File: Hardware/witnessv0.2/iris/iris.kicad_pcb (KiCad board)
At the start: 4 copper layers, 20 x 40 mm, 96 parts, among them J1 Conn_01x02, J2 Conn_01x02, J3 USB_B_Micro, J4 Conn_01x02, J5 Conn_01x04, J6 Conn_01x04, J7 Conn_01x04, J8 Conn_01x04, Q1 SQA403EJ, Q11 AO3400A, Q12 SQA403EJ, Q2 SQA403EJ, Q3 SQA403EJ, Q4 AO3400A, Q5 AO3400A, Q6 SQA403EJ, U1 PAC1934x-xJQ, U2 ME6118A33PG, U3 LTV-817S, U4 MCP23008-xML, U5 TCAN1044A-Q1, U6 TPS63070, U7 ESP32-C3FH4, U9 USBLC6-2SC6, Y1 F322540MUBCE2O

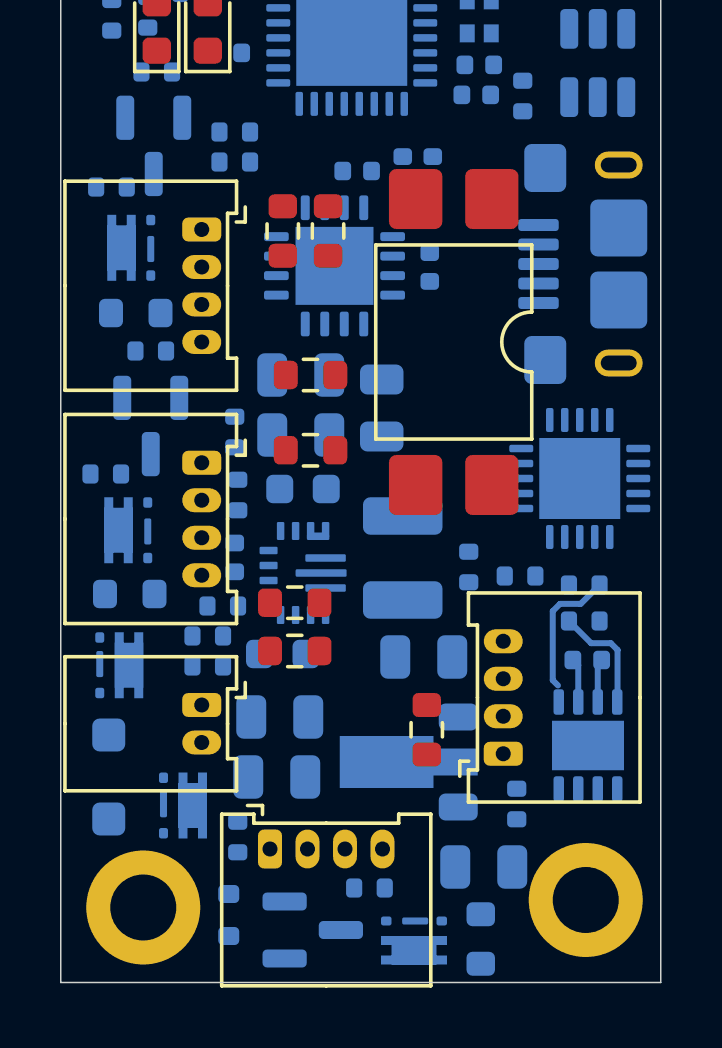
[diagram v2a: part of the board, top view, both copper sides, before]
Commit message: for foo & root
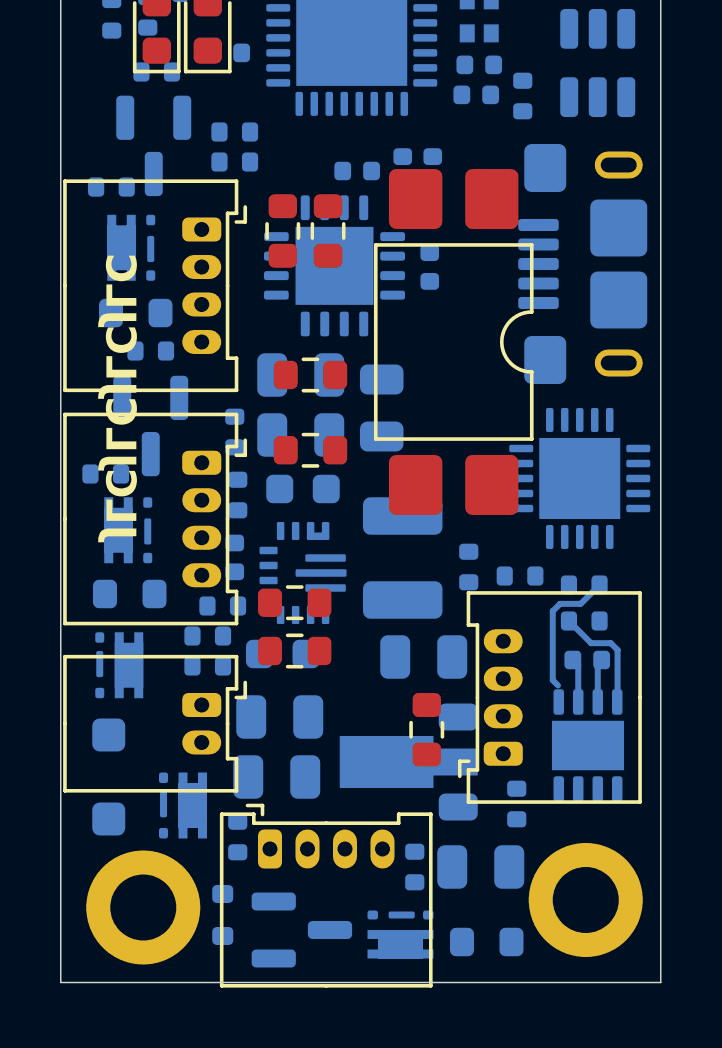
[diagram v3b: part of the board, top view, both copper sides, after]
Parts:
- moved R41 1.66 mm to (114.8, 134.9), turned to 90 degrees
- moved Q6 0.49 mm to (114.3, 137.2)
- moved Q5 0.36 mm to (111.0, 137.0)
- moved R44 0.22 mm to (117.2, 137.4), turned to 180 degrees
- moved D5 0.20 mm to (108.4, 136.5)
- moved C10 0.10 mm to (117.0, 134.9)
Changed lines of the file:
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@@
 	(footprint "Package_TO_SOT_SMD:Vishay_PowerPAK_SC70-6L_Single"
 		(layer "B.Cu")
-		(at 114.775 137.35)
+		(at 114.325 137.15)
 		(descr "Vishay PowerPAK SC70 single transistor package http://www.vishay.com/docs/70486/70486.pdf")
 		(tags "powerpak sc70 sc-70")
@@
 	(footprint "Diode_SMD:D_SOD-523"
 		(layer "B.Cu")
-		(at 108.6 136.5 -90)
+		(at 108.4 136.5 -90)
 		(descr "http://www.diodes.com/datasheets/ap02001.pdf p.144")
 		(tags "Diode SOD523")
@@
 	(footprint "Package_TO_SOT_SMD:SOT-23"
 		(layer "B.Cu")
-		(at 111.4 137)
+		(at 111.0375 137)
 		(descr "SOT, 3 Pin (JEDEC TO-236 Var AB https://www.jedec.org/document_search?search_api_views_fulltext=TO-236)")
 		(tags "SOT TO_SOT_SMD")
@@
 	(footprint "Resistor_SMD:R_0402_1005Metric"
 		(layer "B.Cu")
-		(at 113.29 135.6 180)
+		(at 114.8 134.9 90)
 		(descr "Resistor SMD 0402 (1005 Metric), square (rectangular) end terminal, IPC-7351 nominal, (Body size source: IPC-SM-782 page 72, https://www.pcb-3d.com/wordpress/wp-content/uploads/ipc-sm-782a_amendment_1_and_2.pdf)")
 		(tags "resistor")
 		(property "Reference" "R41"
-			(at 0 1.17 0)
+			(at 0 1.17 90)
 			(layer "B.SilkS")
 			(hide yes)
@@
 		)
 		(property "Value" "1k"
-			(at 0 -1.17 0)
+			(at 0 -1.17 90)
 			(layer "B.Fab")
 			(effects
@@
 		)
 		(property "Datasheet" ""
-			(at 0 0 0)
+			(at 0 0 90)
 			(layer "B.Fab")
 			(hide yes)
@@
 		)
 		(property "Description" "Resistor, small symbol"
-			(at 0 0 0)
+			(at 0 0 90)
 			(layer "B.Fab")
 			(hide yes)
@@
 		)
 		(property "KiLib_Generator" "SMD_2terminal_chip_molded"
-			(at 0 0 0)
+			(at 0 0 90)
 			(layer "B.SilkS")
 			(hide yes)
@@
 		)
 		(property "LCSC_Part" "C11702"
-			(at 0 0 0)
+			(at 0 0 270)
 			(unlocked yes)
 			(layer "B.Fab")
@@
 		(duplicate_pad_numbers_are_jumpers no)
 		(fp_line
-			(start -0.153641 0.38)
-			(end 0.153641 0.38)
+			(start -0.153641 -0.38)
+			(end 0.153641 -0.38)
 			(stroke
 				(width 0.12)
@@
 		)
 		(fp_line
-			(start -0.153641 -0.38)
-			(end 0.153641 -0.38)
+			(start -0.153641 0.38)
+			(end 0.153641 0.38)
 			(stroke
 				(width 0.12)
@@
 		)
 		(fp_text user "${REFERENCE}"
-			(at 0 0 0)
+			(at 0 0 90)
 			(layer "B.Fab")
 			(effects
@@
 		)
 		(pad "1" smd roundrect
-			(at -0.51 0 180)
+			(at -0.51 0 90)
 			(size 0.54 0.64)
 			(layers "B.Cu" "B.Mask" "B.Paste")
@@
 		)
 		(pad "2" smd roundrect
-			(at 0.51 0 180)
+			(at 0.51 0 90)
 			(size 0.54 0.64)
 			(layers "B.Cu" "B.Mask" "B.Paste")
@@
 	(footprint "Capacitor_SMD:C_0805_2012Metric"
 		(layer "B.Cu")
-		(at 117.1 134.9)
+		(at 117 134.9)
 		(descr "Capacitor SMD 0805 (2012 Metric), square (rectangular) end terminal, IPC-7351 nominal, (Body size source: IPC-SM-782 page 76, https://www.pcb-3d.com/wordpress/wp-content/uploads/ipc-sm-782a_amendment_1_and_2.pdf, https://docs.google.com/spreadsheets/d/1BsfQQcO9C6DZCsRaXUlFlo91Tg2WpOkGARC1WS5S8t0/edit?usp=sharing)")
 		(tags "capacitor")
@@
 	(footprint "Resistor_SMD:R_0603_1608Metric"
 		(layer "B.Cu")
-		(at 117 137.3 -90)
+		(at 117.2 137.4 180)
 		(descr "Resistor SMD 0603 (1608 Metric), square (rectangular) end terminal, IPC-7351 nominal, (Body size source: IPC-SM-782 page 72, https://www.pcb-3d.com/wordpress/wp-content/uploads/ipc-sm-782a_amendment_1_and_2.pdf)")
 		(tags "resistor")
 		(property "Reference" "R44"
-			(at 0 1.43 90)
+			(at 0 1.43 0)
 			(layer "B.SilkS")
 			(hide yes)
@@
 		)
 		(property "Value" "20m"
-			(at 0 -1.43 90)
+			(at 0 -1.43 0)
 			(layer "B.Fab")
 			(effects
@@
 		)
 		(property "Datasheet" ""
-			(at 0 0 90)
+			(at 0 0 0)
 			(layer "B.Fab")
 			(hide yes)
@@
 		)
 		(property "Description" "Resistor, small symbol"
-			(at 0 0 90)
+			(at 0 0 0)
 			(layer "B.Fab")
 			(hide yes)
@@
 		)
 		(property "KiLib_Generator" "SMD_2terminal_chip_molded"
-			(at 0 0 90)
+			(at 0 0 0)
 			(layer "B.SilkS")
 			(hide yes)
@@
 		)
 		(property "LCSC_Part" ""
-			(at 0 0 90)
+			(at 0 0 0)
 			(unlocked yes)
 			(layer "B.Fab")
@@
 		)
 		(fp_text user "${REFERENCE}"
-			(at 0 0 90)
+			(at 0 0 0)
 			(layer "B.Fab")
 			(effects
@@
 		)
 		(pad "1" smd roundrect
-			(at -0.825 0 270)
+			(at -0.825 0 180)
 			(size 0.8 0.95)
 			(layers "B.Cu" "B.Mask" "B.Paste")
@@
 		)
 		(pad "2" smd roundrect
-			(at 0.825 0 270)
+			(at 0.825 0 180)
 			(size 0.8 0.95)
 			(layers "B.Cu" "B.Mask" "B.Paste")
@@
 	)
 	(gr_text "JLCJLCJLCJLC"
-		(at 108 138.4 0)
-		(layer "B.SilkS")
+		(at 104.4 124 270)
+		(layer "F.SilkS")
 		(effects
 			(font
@@
 				(bold yes)
 			)
-			(justify left bottom)
+			(justify left bottom mirror)
 		)
 	)

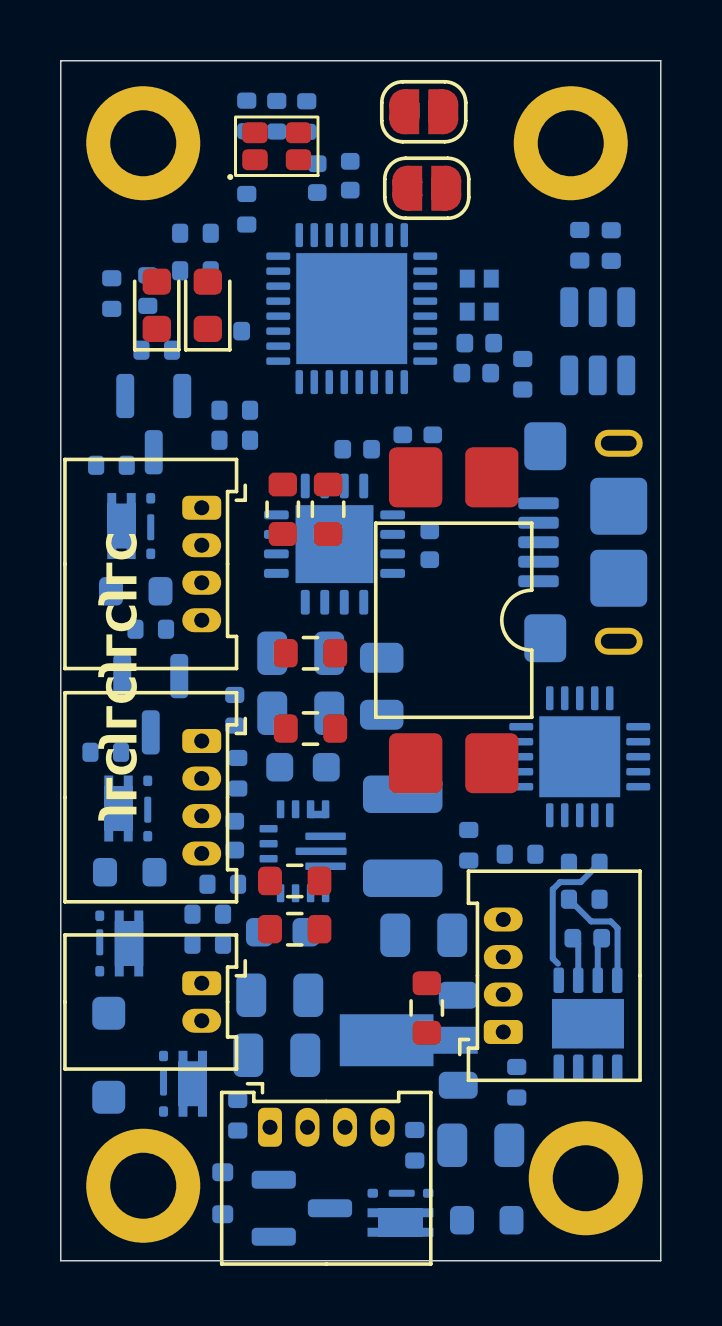
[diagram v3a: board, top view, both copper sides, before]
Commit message: routed
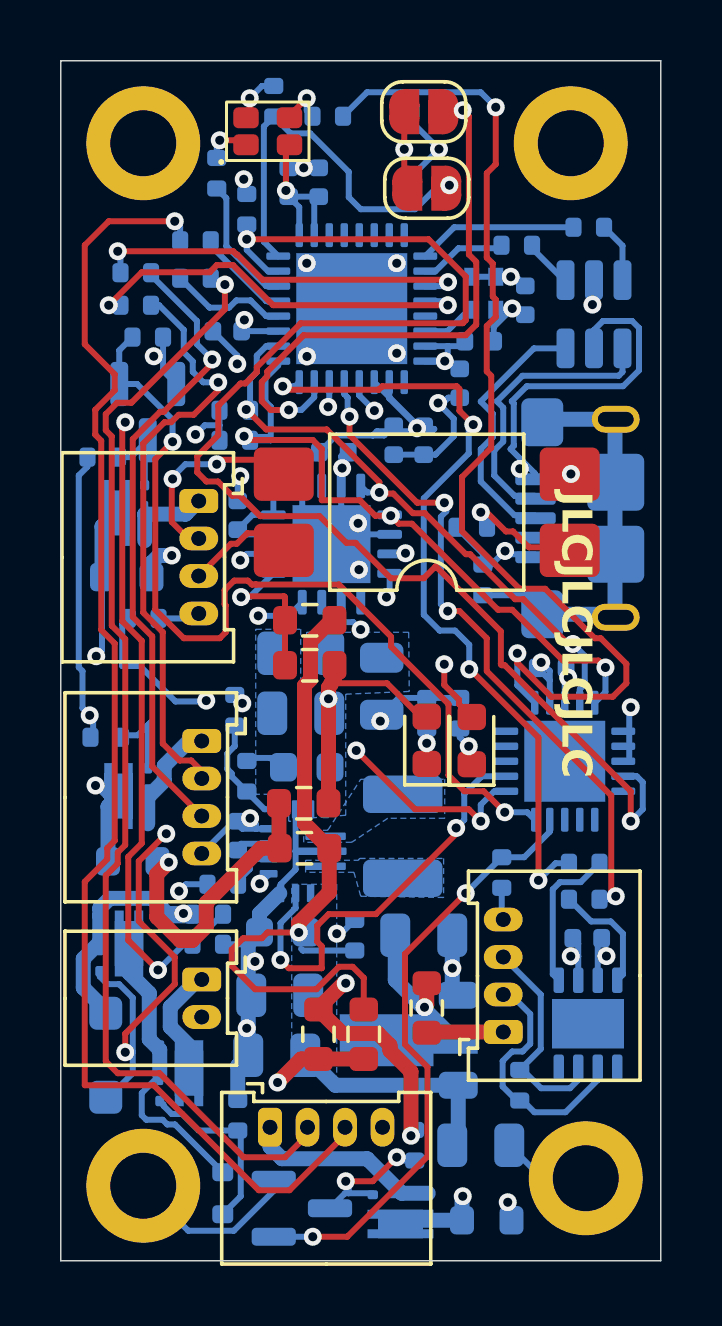
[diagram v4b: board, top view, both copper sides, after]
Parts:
- removed Q4: AO3400A, Package_TO_SOT_SMD:SOT-23
- added C29: 100n, Capacitor_SMD:C_0402_1005Metric, B.Cu at (119.4, 119.0)
- added C30: 100n, Capacitor_SMD:C_0402_1005Metric, B.Cu at (118.5, 106.7)
- added R37: 0, Resistor_SMD:R_0402_1005Metric, B.Cu at (105.5, 106.9)
- added R47: 0, Resistor_SMD:R_0402_1005Metric, B.Cu at (117.1, 116.1)
- added R50: 0, Resistor_SMD:R_0402_1005Metric, B.Cu at (105.5, 105.8)
- moved R20 18.2 mm to (116.3, 120.5)
- moved D2 17.9 mm to (116.7, 121.4)
- moved R1 17.7 mm to (113.1, 131.2), turned to -90 degrees
- moved R2 17.5 mm to (111.6, 131.2), turned to -90 degrees
- moved R38 16.9 mm to (115.2, 120.5)
- moved D3 16.2 mm to (115.2, 121.4)
- moved R3 10.3 mm to (111.3, 117.4)
- moved Q12 9.85 mm to (105.2, 113.8)
- moved R48 9.84 mm to (104.4, 112.0)
- moved R49 9.84 mm to (105.2, 116.0)
- moved Q11 9.74 mm to (105.9, 110.5)
- moved R53 9.74 mm to (105.9, 108.0)
- moved R40 9.07 mm to (104.5, 121.3)
- moved Q3 9.00 mm to (105.2, 123.3)
- moved R43 9.00 mm to (105.4, 125.4)
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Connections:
- J3 pad SH: unconnected-(J3-Shield-PadSH)_2 -> Net-(J3-Shield)
- U1 pad 11: /Load Switches/VIN1 -> /Load Switches/VIN3
- U1 pad 12: /Load Switches/CS1 -> /Load Switches/CS3
- U1 pad 13: /Load Switches/VIN1 -> /Load Switches/VIN2
- U1 pad 16: GND -> +3V3
- U1 pad 7: /Load Switches/CS3 -> /Load Switches/CS1
- U3 pad 1: /IO/BUTTON -> Net-(R46-Pad1)
- U3 pad 2: Net-(R46-Pad1) -> /IO/BUTTON
- U3 pad 3: Net-(J8-Pin_3) -> Net-(J8-Pin_2)
- U3 pad 4: Net-(J8-Pin_2) -> Net-(J8-Pin_3)
- U7 pad 15: /MCU/LED_G -> /MCU/LS_EN
- U7 pad 16: /MCU/LS_EN -> /MCU/LED_G
- U7 pad 27: /IO/RXD0_MCU -> /MCU/RXD0_MCU
- U7 pad 28: /IO/TXD0_MCU -> /MCU/TXD0_MCU
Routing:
- net GND: track 1.47 -> 61.4 mm, vias 0 -> 25
- net +5V: track 0.00 -> 54.7 mm, vias 0 -> 6
- net VBUS: track 0.00 -> 47.4 mm, vias 0 -> 3
- net /MCU/LS_EN: track 0.00 -> 46.6 mm, vias 0 -> 2
- net /IO/RXD1_MCU: track 0.00 -> 44.3 mm, vias 0 -> 1
- net +BATT: track 0.00 -> 42.2 mm, vias 0 -> 2
- net +3V3: track 1.45 -> 42.2 mm, vias 0 -> 11
- net /IO/TXD1_MCU: track 0.00 -> 37.3 mm, vias 0 -> 1
- net /MCU/VSENSE: track 0.00 -> 35.4 mm, vias 0 -> 3
- net /MCU/LED_B: track 0.00 -> 35.1 mm, vias 0 -> 2
- net /Load Switches/CS1: track 0.00 -> 34.2 mm, vias 0 -> 2
- net /Load Switches/VIN1: track 0.00 -> 31.1 mm, vias 0 -> 3
- net /Load Switches/EN2: track 0.00 -> 30.2 mm, vias 0 -> 2
- net /Load Switches/VIN3: track 0.00 -> 27.3 mm, vias 0 -> 2
- net /MCU/CANRX: track 0.00 -> 27.0 mm, vias 0 -> 4
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- added copper zone on B.Cu, net +5V
- added copper zone on B.Cu, net +BATT
- added copper zone on B.Cu, net GND
- added copper zone on B.Cu, net Net-(U6-L1)
- added copper zone on B.Cu, net Net-(U6-L2)
